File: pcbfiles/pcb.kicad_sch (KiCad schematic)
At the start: 236 parts, among them J1 Conn_01x06, J2 Conn_01x06, J3 Conn_01x06, J4 Conn_01x06, J5 Conn_01x04_Female, J6 Conn_01x04_Female, Q1 AO3401A, Q2 AO3401A, SW1 SW_SPST, SW10 SW_SPST, SW11 SW_SPST, SW12 SW_SPST, SW13 SW_SPST, SW14 SW_SPST, SW15 SW_SPST, SW16 SW_SPST, SW17 SW_SPST, SW18 SW_SPST, SW19 SW_SPST, SW2 SW_SPST, SW20 SW_SPST, SW21 SW_SPST, SW22 SW_SPST, SW23 SW_SPST, SW24 SW_SPST, SW25 SW_SPST, SW26 SW_SPST, SW27 SW_SPST, SW28 SW_SPST, SW29 SW_SPST, SW3 SW_SPST, SW30 SW_SPST, SW31 SW_SPST, SW32 SW_SPST, SW33 SW_SPST, SW34 SW_SPST, SW35 SW_SPST, SW36 SW_SPST, SW37 SW_SPST, SW38 SW_SPST, SW39 SW_SPST, SW4 SW_SPST, SW40 SW_SPST, SW41 SW_SPST, SW42 SW_SPST, SW43 SW_SPST, SW44 SW_SPST, SW45 SW_SPST, SW46 SW_SPST, SW47 SW_SPST, SW48 SW_SPST, SW49 SW_SPST, SW5 SW_SPST, SW50 SW_SPST, SW51 SW_SPST, SW52 SW_SPST, SW53 SW_SPST, SW54 SW_SPST, SW55 SW_SPST, SW56 SW_SPST, SW57 SW_SPST, SW58 SW_SPST, SW59 SW_SPST, SW6 SW_SPST, SW60 SW_SPST, SW61 SW_SPST, SW62 SW_SPST, SW63 SW_SPST, SW64 SW_SPST, SW65 SW_SPST, SW66 SW_SPST, SW67 SW_SPST, SW68 SW_SPST, SW69 SW_SPST, SW7 SW_SPST, SW70 SW_SPST, SW71 SW_SPST, SW72 SW_SPST, SW73 SW_SPST, SW74 SW_SPST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

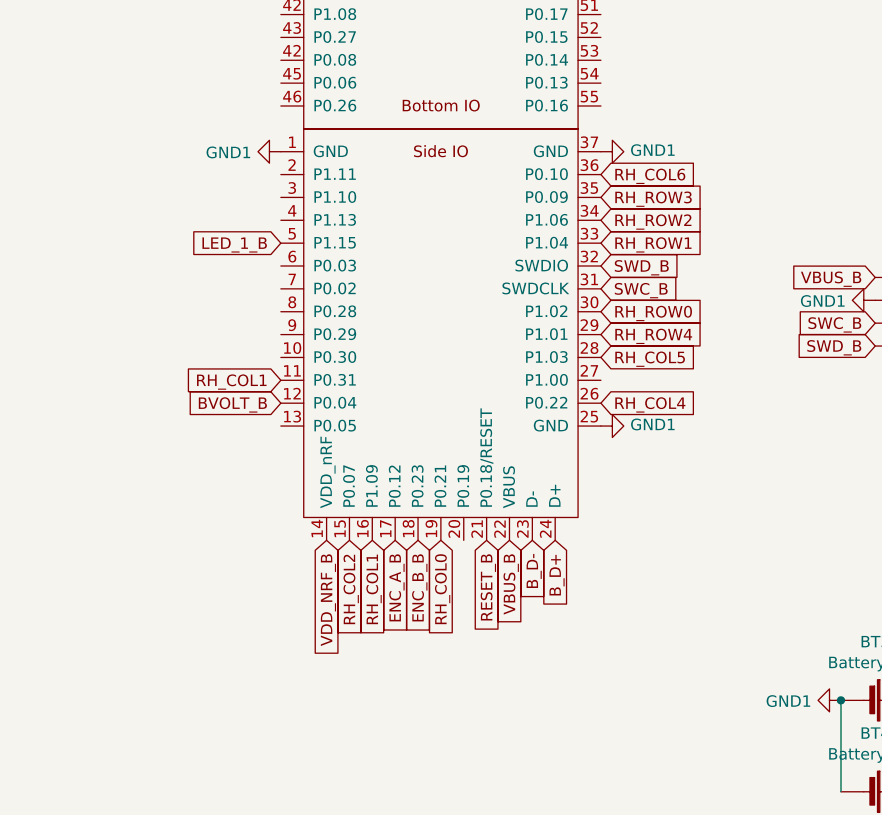
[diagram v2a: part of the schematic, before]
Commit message: I'm so close I can feel it.
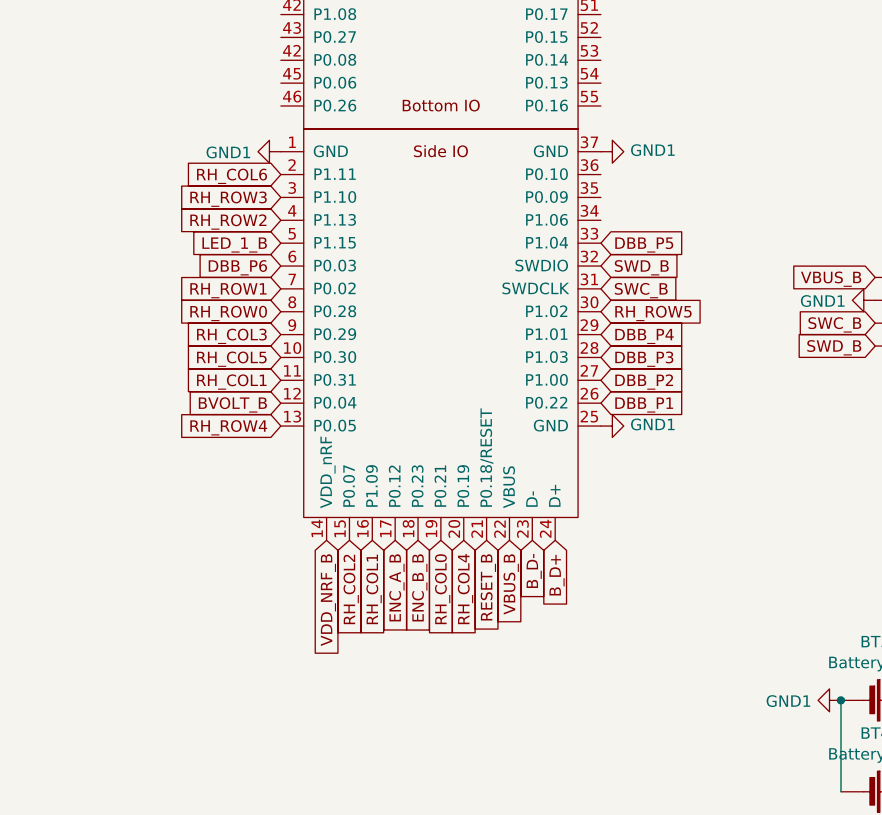
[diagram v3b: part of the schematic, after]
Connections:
- net DBB_P1: now also U6.26 (P0.22)
- net DBB_P2: now also U6.27 (P1.00)
- net DBB_P3: now also U6.28 (P1.03)
- net DBB_P4: now also U6.29 (P1.01)
- net DBB_P5: now also U6.33 (P1.04)
- net DBB_P6: now also U6.6 (P0.03)
- net RH_COL3: now also U6.9 (P0.29)
- net RH_COL4: now also U6.20 (P0.19); no longer U6.26 (P0.22)
- net RH_COL5: now also U6.10 (P0.30); no longer U6.28 (P1.03)
- net RH_COL6: now also U6.2 (P1.11); no longer U6.36 (P0.10)
- net RH_ROW0: now also U6.8 (P0.28); no longer U6.30 (P1.02)
- net RH_ROW1: now also U6.7 (P0.02); no longer U6.33 (P1.04)
- net RH_ROW2: now also U6.4 (P1.13); no longer U6.34 (P1.06)
- net RH_ROW3: now also U6.3 (P1.10); no longer U6.35 (P0.09)
- net RH_ROW4: now also U6.13 (P0.05); no longer U6.29 (P1.01)
- net RH_ROW5: now also U6.30 (P1.02)
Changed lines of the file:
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@@
+    )
+  )
+  (global_label "RH_ROW4" (shape input) (at 489.712 275.59 180) (fields_autoplaced)
+    (effects (font (size 1.27 1.27)) (justify right))
+    (property "Intersheet References" "${INTERSHEET_REFS}" (id 0) (at 478.5583 275.5106 0)
+      (effects (font (size 1.27 1.27)) (justify right) hide)
     )
   )
@@
     )
   )
+  (global_label "DBB_P1" (shape input) (at 525.272 273.05 0) (fields_autoplaced)
+    (effects (font (size 1.27 1.27)) (justify left))
+    (property "Intersheet References" "${INTERSHEET_REFS}" (id 0) (at 534.8533 273.1294 0)
+      (effects (font (size 1.27 1.27)) (justify left) hide)
+    )
+  )
   (global_label "D+" (shape input) (at 74.422 181.61 0) (fields_autoplaced)
     (effects (font (size 1.27 1.27)) (justify left))
@@
     (property "Intersheet References" "${INTERSHEET_REFS}" (id 0) (at 13.462 128.27 0)
       (effects (font (size 1.27 1.27)) hide)
+    )
+  )
+  (global_label "RH_ROW5" (shape input) (at 525.272 262.89 0) (fields_autoplaced)
+    (effects (font (size 1.27 1.27)) (justify left))
+    (property "Intersheet References" "${INTERSHEET_REFS}" (id 0) (at 536.4257 262.8106 0)
+      (effects (font (size 1.27 1.27)) (justify left) hide)
     )
   )
@@
     )
   )
-  (global_label "RH_ROW4" (shape input) (at 525.272 265.43 0) (fields_autoplaced)
-    (effects (font (size 1.27 1.27)) (justify left))
-    (property "Intersheet References" "${INTERSHEET_REFS}" (id 0) (at 536.4257 265.3506 0)
-      (effects (font (size 1.27 1.27)) (justify left) hide)
+  (global_label "DBB_P2" (shape input) (at 525.272 270.51 0) (fields_autoplaced)
+    (effects (font (size 1.27 1.27)) (justify left))
+    (property "Intersheet References" "${INTERSHEET_REFS}" (id 0) (at 534.8533 270.5894 0)
+      (effects (font (size 1.27 1.27)) (justify left) hide)
+    )
+  )
+  (global_label "RH_COL3" (shape input) (at 489.712 265.43 180) (fields_autoplaced)
+    (effects (font (size 1.27 1.27)) (justify right))
+    (property "Intersheet References" "${INTERSHEET_REFS}" (id 0) (at 478.9816 265.3506 0)
+      (effects (font (size 1.27 1.27)) (justify right) hide)
     )
   )
@@
     )
   )
-  (global_label "RH_COL5" (shape input) (at 525.272 267.97 0) (fields_autoplaced)
-    (effects (font (size 1.27 1.27)) (justify left))
-    (property "Intersheet References" "${INTERSHEET_REFS}" (id 0) (at 536.0024 267.8906 0)
-      (effects (font (size 1.27 1.27)) (justify left) hide)
+  (global_label "RH_COL5" (shape input) (at 489.712 267.97 180) (fields_autoplaced)
+    (effects (font (size 1.27 1.27)) (justify right))
+    (property "Intersheet References" "${INTERSHEET_REFS}" (id 0) (at 478.9816 267.8906 0)
+      (effects (font (size 1.27 1.27)) (justify right) hide)
     )
   )
@@
     )
   )
-  (global_label "RH_ROW2" (shape input) (at 525.272 252.73 0) (fields_autoplaced)
-    (effects (font (size 1.27 1.27)) (justify left))
-    (property "Intersheet References" "${INTERSHEET_REFS}" (id 0) (at -130.048 133.35 0)
+  (global_label "RH_ROW2" (shape input) (at 489.712 252.73 180) (fields_autoplaced)
+    (effects (font (size 1.27 1.27)) (justify right))
+    (property "Intersheet References" "${INTERSHEET_REFS}" (id 0) (at 1145.032 372.11 0)
       (effects (font (size 1.27 1.27)) hide)
     )
@@
     )
   )
-  (global_label "RH_ROW1" (shape input) (at 525.272 255.27 0) (fields_autoplaced)
-    (effects (font (size 1.27 1.27)) (justify left))
-    (property "Intersheet References" "${INTERSHEET_REFS}" (id 0) (at 536.4257 255.1906 0)
-      (effects (font (size 1.27 1.27)) (justify left) hide)
+  (global_label "RH_ROW1" (shape input) (at 489.712 260.35 180) (fields_autoplaced)
+    (effects (font (size 1.27 1.27)) (justify right))
+    (property "Intersheet References" "${INTERSHEET_REFS}" (id 0) (at 478.5583 260.4294 0)
+      (effects (font (size 1.27 1.27)) (justify right) hide)
     )
   )
@@
     (property "Intersheet References" "${INTERSHEET_REFS}" (id 0) (at 60.452 128.27 0)
       (effects (font (size 1.27 1.27)) hide)
+    )
+  )
+  (global_label "DBB_P4" (shape input) (at 525.272 265.43 0) (fields_autoplaced)
+    (effects (font (size 1.27 1.27)) (justify left))
+    (property "Intersheet References" "${INTERSHEET_REFS}" (id 0) (at 534.8533 265.3506 0)
+      (effects (font (size 1.27 1.27)) (justify left) hide)
     )
   )
@@
     )
   )
-  (global_label "RH_COL4" (shape input) (at 525.272 273.05 0) (fields_autoplaced)
-    (effects (font (size 1.27 1.27)) (justify left))
-    (property "Intersheet References" "${INTERSHEET_REFS}" (id 0) (at 609.092 -336.55 0)
+  (global_label "RH_COL4" (shape input) (at 510.032 288.29 270) (fields_autoplaced)
+    (effects (font (size 1.27 1.27)) (justify right))
+    (property "Intersheet References" "${INTERSHEET_REFS}" (id 0) (at 1119.632 372.11 0)
       (effects (font (size 1.27 1.27)) hide)
     )
@@
     )
   )
-  (global_label "RH_ROW3" (shape input) (at 525.272 250.19 0) (fields_autoplaced)
-    (effects (font (size 1.27 1.27)) (justify left))
-    (property "Intersheet References" "${INTERSHEET_REFS}" (id 0) (at -130.048 120.65 0)
+  (global_label "RH_ROW3" (shape input) (at 489.712 250.19 180) (fields_autoplaced)
+    (effects (font (size 1.27 1.27)) (justify right))
+    (property "Intersheet References" "${INTERSHEET_REFS}" (id 0) (at 1145.032 379.73 0)
       (effects (font (size 1.27 1.27)) hide)
     )
@@
     (property "Intersheet References" "${INTERSHEET_REFS}" (id 0) (at 9.652 128.27 0)
       (effects (font (size 1.27 1.27)) hide)
+    )
+  )
+  (global_label "DBB_P5" (shape input) (at 525.272 255.27 0) (fields_autoplaced)
+    (effects (font (size 1.27 1.27)) (justify left))
+    (property "Intersheet References" "${INTERSHEET_REFS}" (id 0) (at 534.8533 255.3494 0)
+      (effects (font (size 1.27 1.27)) (justify left) hide)
     )
   )
@@
     )
   )
-  (global_label "RH_ROW0" (shape input) (at 525.272 262.89 0) (fields_autoplaced)
-    (effects (font (size 1.27 1.27)) (justify left))
-    (property "Intersheet References" "${INTERSHEET_REFS}" (id 0) (at 536.4257 262.8106 0)
-      (effects (font (size 1.27 1.27)) (justify left) hide)
+  (global_label "RH_ROW0" (shape input) (at 489.712 262.89 180) (fields_autoplaced)
+    (effects (font (size 1.27 1.27)) (justify right))
+    (property "Intersheet References" "${INTERSHEET_REFS}" (id 0) (at 478.5583 262.9694 0)
+      (effects (font (size 1.27 1.27)) (justify right) hide)
+    )
+  )
+  (global_label "DBB_P6" (shape input) (at 489.712 257.81 180) (fields_autoplaced)
+    (effects (font (size 1.27 1.27)) (justify right))
+    (property "Intersheet References" "${INTERSHEET_REFS}" (id 0) (at 480.1307 257.7306 0)
+      (effects (font (size 1.27 1.27)) (justify right) hide)
     )
   )
@@
     (property "Intersheet References" "${INTERSHEET_REFS}" (id 0) (at 9.652 128.27 0)
       (effects (font (size 1.27 1.27)) hide)
+    )
+  )
+  (global_label "DBB_P3" (shape input) (at 525.272 267.97 0) (fields_autoplaced)
+    (effects (font (size 1.27 1.27)) (justify left))
+    (property "Intersheet References" "${INTERSHEET_REFS}" (id 0) (at 534.8533 268.0494 0)
+      (effects (font (size 1.27 1.27)) (justify left) hide)
     )
   )
@@
     )
   )
-  (global_label "RH_COL6" (shape input) (at 525.272 247.65 0) (fields_autoplaced)
-    (effects (font (size 1.27 1.27)) (justify left))
-    (property "Intersheet References" "${INTERSHEET_REFS}" (id 0) (at 609.092 -397.51 0)
-      (effects (font (size 1.27 1.27)) hide)
-    )
+  (global_label "RH_COL6" (shape input) (at 489.712 247.65 180) (fields_autoplaced)
+    (effects (font (size 1.27 1.27)) (justify right))
+    (property "Intersheet References" "${INTERSHEET_REFS}" (id 0) (at 405.892 892.81 0)
+      (effects (font (size 1.27 1.27)) hide)
+    )

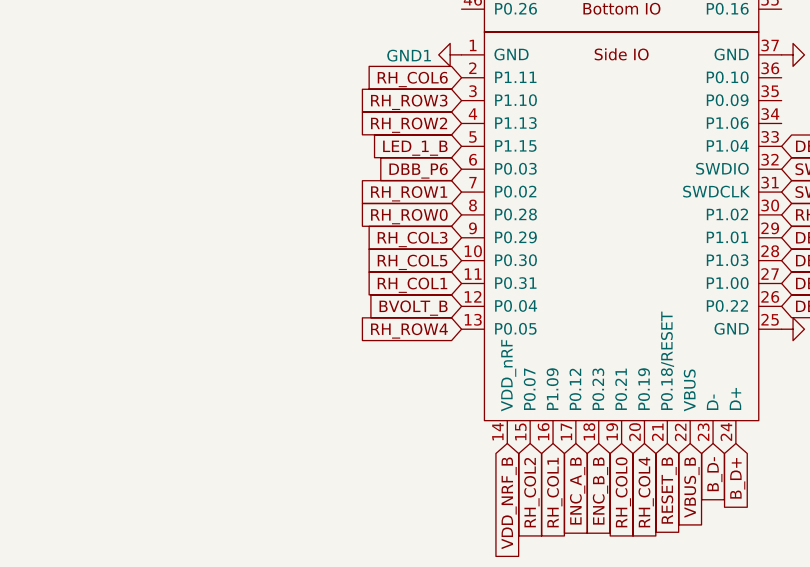
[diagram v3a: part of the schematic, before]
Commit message: Routing.
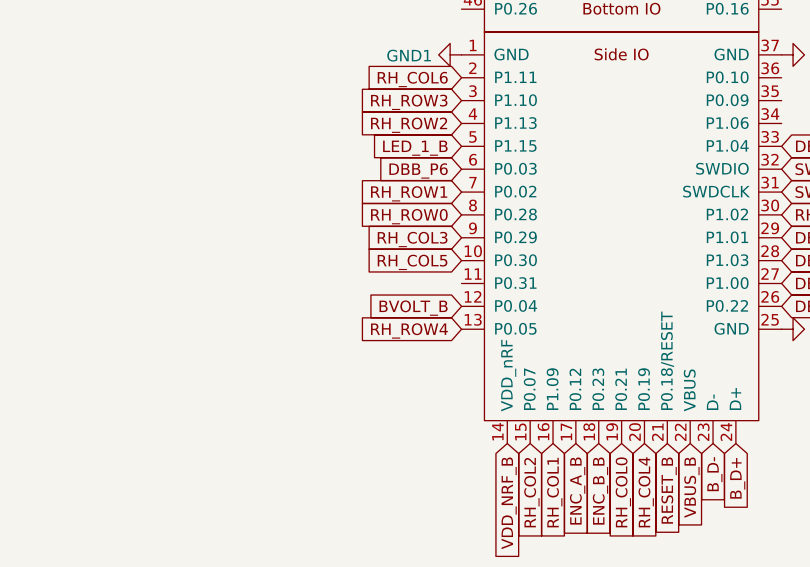
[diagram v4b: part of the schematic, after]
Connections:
- net RH_COL1: no longer U6.11 (P0.31)
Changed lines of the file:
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@@
-    )
-  )
-  (global_label "RH_COL1" (shape input) (at 489.712 270.51 180) (fields_autoplaced)
-    (effects (font (size 1.27 1.27)) (justify right))
-    (property "Intersheet References" "${INTERSHEET_REFS}" (id 0) (at 405.892 826.77 0)
-      (effects (font (size 1.27 1.27)) hide)
     )
   )

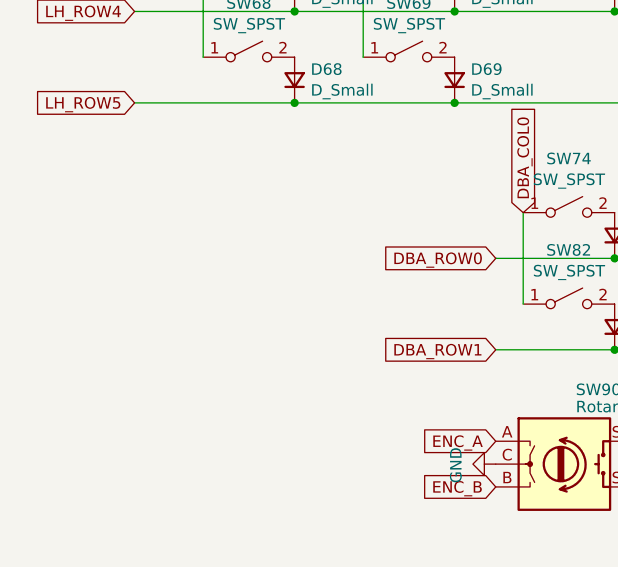
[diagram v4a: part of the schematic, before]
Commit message: Routing.
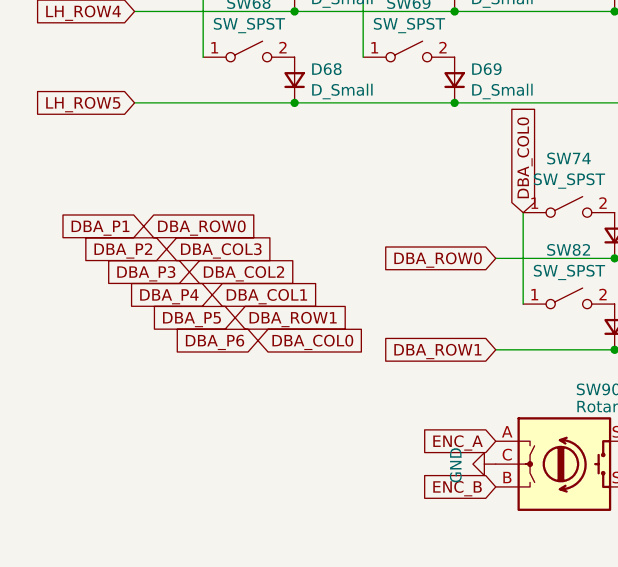
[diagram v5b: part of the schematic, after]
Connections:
- net DBA_P2 is gone; now on net DBA_COL3: J1.2 (Pin_2), J3.5 (Pin_5), U5.10 (P0.30)
- net DBA_P3 is gone; now on net DBA_COL2: J1.3 (Pin_3), J3.4 (Pin_4), U5.9 (P0.29)
- net DBA_P4 is gone; now on net DBA_COL1: J1.4 (Pin_4), J3.3 (Pin_3), U5.8 (P0.28)
- net DBA_P6 is gone; now on net DBA_COL0: J1.6 (Pin_6), J3.1 (Pin_1), U5.6 (P0.03)
- net DBA_ROW0 is gone; now on net DBA_P1: D74.1 (K), D75.1 (K), D76.1 (K), D77.1 (K)
- net DBA_ROW1 is gone; now on net DBA_P5: D82.1 (K), D83.1 (K), D84.1 (K), D85.1 (K)
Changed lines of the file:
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@@
+    )
+  )
+  (global_label "DBA_ROW1" (shape input) (at 37.846 115.316 0) (fields_autoplaced)
+    (effects (font (size 1.27 1.27)) (justify left))
+    (property "Intersheet References" "${INTERSHEET_REFS}" (id 0) (at 50.0278 115.3954 0)
+      (effects (font (size 1.27 1.27)) (justify left) hide)
     )
   )
@@
     )
   )
+  (global_label "DBA_COL0" (shape input) (at 40.386 117.856 0) (fields_autoplaced)
+    (effects (font (size 1.27 1.27)) (justify left))
+    (property "Intersheet References" "${INTERSHEET_REFS}" (id 0) (at 52.1445 117.7766 0)
+      (effects (font (size 1.27 1.27)) (justify left) hide)
+    )
+  )
   (global_label "RAW" (shape input) (at 111.252 153.67 180) (fields_autoplaced)
     (effects (font (size 1.27 1.27)) (justify right))
@@
     )
   )
+  (global_label "DBA_COL3" (shape input) (at 30.226 107.696 0) (fields_autoplaced)
+    (effects (font (size 1.27 1.27)) (justify left))
+    (property "Intersheet References" "${INTERSHEET_REFS}" (id 0) (at 41.9845 107.6166 0)
+      (effects (font (size 1.27 1.27)) (justify left) hide)
+    )
+  )
   (global_label "ENC_A" (shape input) (at 66.802 129.032 180) (fields_autoplaced)
     (effects (font (size 1.27 1.27)) (justify right))
@@
     )
   )
+  (global_label "DBA_P6" (shape input) (at 40.386 117.856 180) (fields_autoplaced)
+    (effects (font (size 1.27 1.27)) (justify right))
+    (property "Intersheet References" "${INTERSHEET_REFS}" (id 0) (at 30.9861 117.7766 0)
+      (effects (font (size 1.27 1.27)) (justify right) hide)
+    )
+  )
   (global_label "LH_COL0" (shape input) (at 71.882 255.27 0) (fields_autoplaced)
     (effects (font (size 1.27 1.27)) (justify left))
@@
     )
   )
+  (global_label "DBA_ROW0" (shape input) (at 27.686 105.156 0) (fields_autoplaced)
+    (effects (font (size 1.27 1.27)) (justify left))
+    (property "Intersheet References" "${INTERSHEET_REFS}" (id 0) (at 39.8678 105.2354 0)
+      (effects (font (size 1.27 1.27)) (justify left) hide)
+    )
+  )
   (global_label "DBB_COL0" (shape input) (at 501.142 103.886 90) (fields_autoplaced)
     (effects (font (size 1.27 1.27)) (justify left))
@@
     (effects (font (size 1.27 1.27)) (justify right))
     (property "Intersheet References" "${INTERSHEET_REFS}" (id 0) (at 157.7321 108.3786 0)
+      (effects (font (size 1.27 1.27)) (justify right) hide)
+    )
+  )
+  (global_label "DBA_P2" (shape input) (at 30.226 107.696 180) (fields_autoplaced)
+    (effects (font (size 1.27 1.27)) (justify right))
+    (property "Intersheet References" "${INTERSHEET_REFS}" (id 0) (at 20.8261 107.6166 0)
       (effects (font (size 1.27 1.27)) (justify right) hide)
     )
@@
     )
   )
+  (global_label "DBA_P5" (shape input) (at 37.846 115.316 180) (fields_autoplaced)
+    (effects (font (size 1.27 1.27)) (justify right))
+    (property "Intersheet References" "${INTERSHEET_REFS}" (id 0) (at 28.4461 115.2366 0)
+      (effects (font (size 1.27 1.27)) (justify right) hide)
+    )
+  )
   (global_label "RH_COL1" (shape input) (at 501.142 25.654 90) (fields_autoplaced)
     (effects (font (size 1.27 1.27)) (justify left))
@@
     (effects (font (size 1.27 1.27)) (justify right))
     (property "Intersheet References" "${INTERSHEET_REFS}" (id 0) (at 485.7308 108.8866 0)
+      (effects (font (size 1.27 1.27)) (justify right) hide)
+    )
+  )
+  (global_label "DBA_P4" (shape input) (at 35.306 112.776 180) (fields_autoplaced)
+    (effects (font (size 1.27 1.27)) (justify right))
+    (property "Intersheet References" "${INTERSHEET_REFS}" (id 0) (at 25.9061 112.6966 0)
       (effects (font (size 1.27 1.27)) (justify right) hide)
     )
@@
     )
   )
+  (global_label "DBA_COL1" (shape input) (at 35.306 112.776 0) (fields_autoplaced)
+    (effects (font (size 1.27 1.27)) (justify left))
+    (property "Intersheet References" "${INTERSHEET_REFS}" (id 0) (at 47.0645 112.6966 0)
+      (effects (font (size 1.27 1.27)) (justify left) hide)
+    )
+  )
   (global_label "LH_ROW3" (shape input) (at 26.67 71.12 180) (fields_autoplaced)
     (effects (font (size 1.27 1.27)) (justify right))
@@
     )
   )
+  (global_label "DBA_COL2" (shape input) (at 32.766 110.236 0) (fields_autoplaced)
+    (effects (font (size 1.27 1.27)) (justify left))
+    (property "Intersheet References" "${INTERSHEET_REFS}" (id 0) (at 44.5245 110.1566 0)
+      (effects (font (size 1.27 1.27)) (justify left) hide)
+    )
+  )
   (global_label "DBA_P1" (shape input) (at 36.322 270.51 180) (fields_autoplaced)
     (effects (font (size 1.27 1.27)) (justify right))
@@
     )
   )
+  (global_label "DBA_P1" (shape input) (at 27.686 105.156 180) (fields_autoplaced)
+    (effects (font (size 1.27 1.27)) (justify right))
+    (property "Intersheet References" "${INTERSHEET_REFS}" (id 0) (at 18.2861 105.0766 0)
+      (effects (font (size 1.27 1.27)) (justify right) hide)
+    )
+  )
   (global_label "ENC_B" (shape input) (at 66.802 134.112 180) (fields_autoplaced)
     (effects (font (size 1.27 1.27)) (justify right))
@@
     )
   )
+  (global_label "DBA_P3" (shape input) (at 32.766 110.236 180) (fields_autoplaced)
+    (effects (font (size 1.27 1.27)) (justify right))
+    (property "Intersheet References" "${INTERSHEET_REFS}" (id 0) (at 23.3661 110.1566 0)
+      (effects (font (size 1.27 1.27)) (justify right) hide)
+    )
+  )
